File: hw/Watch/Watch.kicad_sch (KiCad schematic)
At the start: 8 parts, among them J3 Conn_01x02, J4 Conn_01x02, J5 Conn_01x02, J6 Conn_01x02

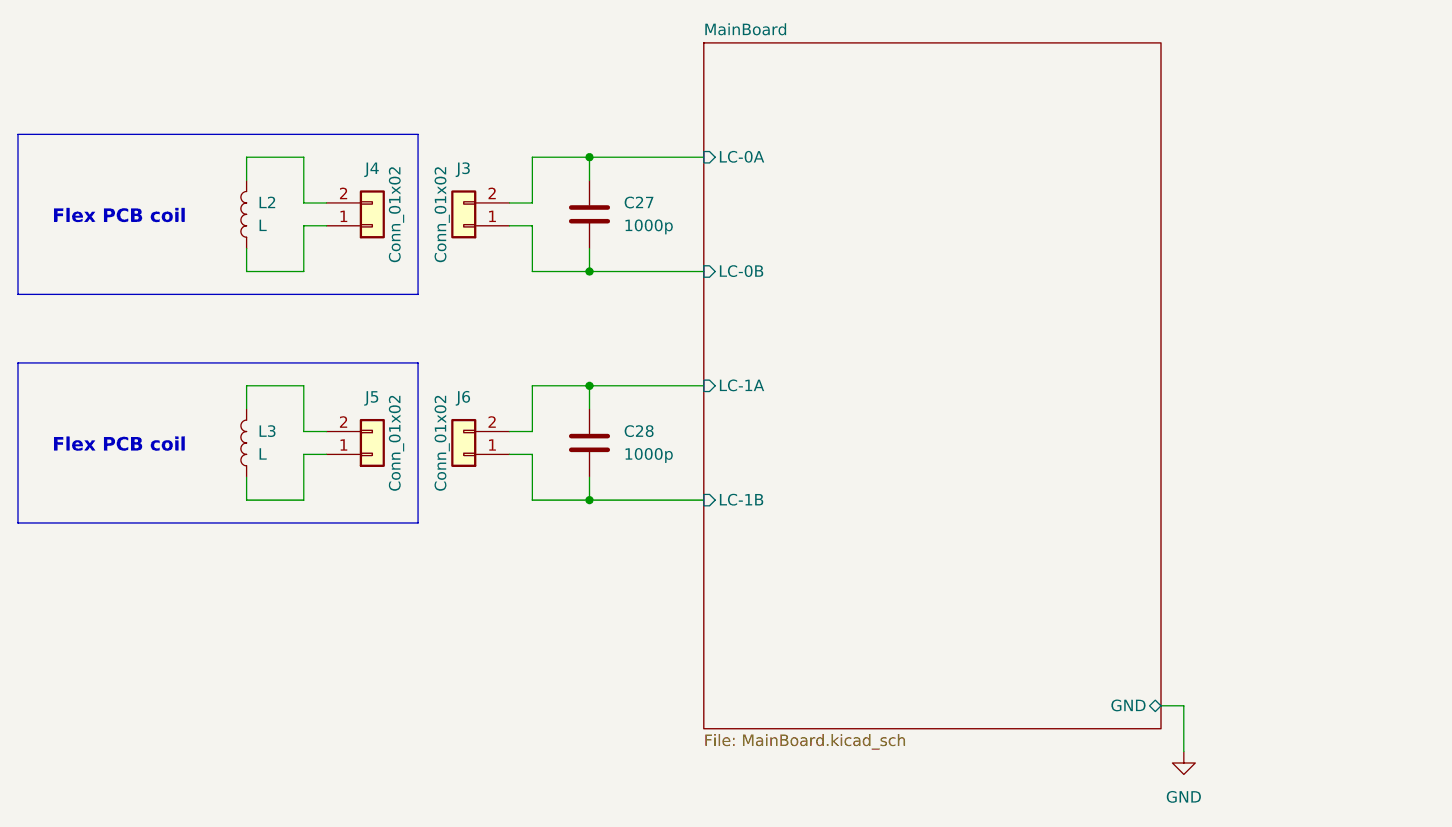
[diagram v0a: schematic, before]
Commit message: wip
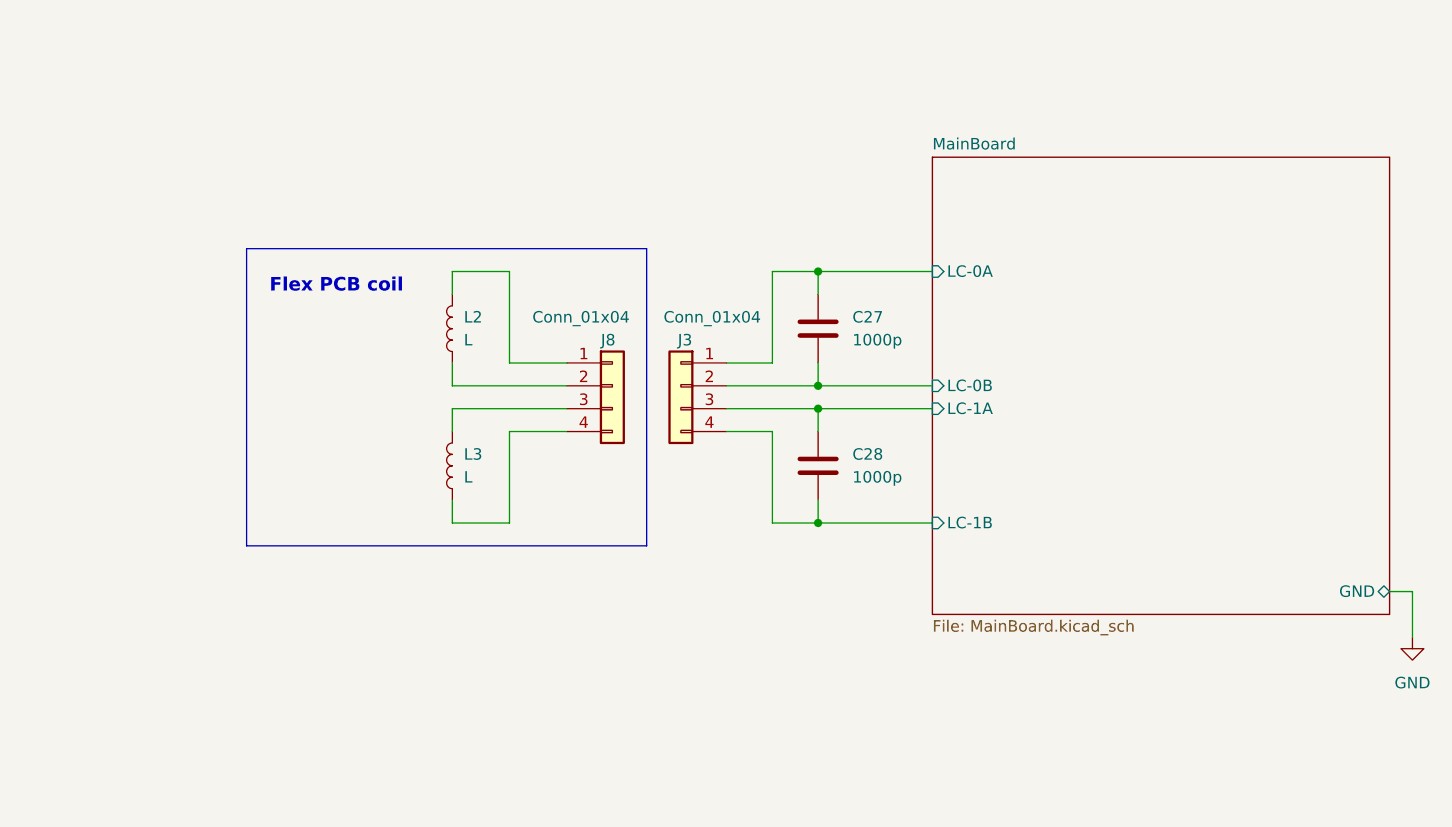
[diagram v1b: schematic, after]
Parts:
- removed J3, J4, J5, J6: Conn_01x02, symbol Connector_Generic:Conn_01x02
- added J3: Conn_01x04, RKL-Connectors:FFC-FPC_1x04_0.5mm, symbol Connector_Generic:Conn_01x04
- added J8: Conn_01x04, RKL-Connectors:FFC-FPC_1x04_0.5mm_cable, symbol Connector_Generic:Conn_01x04
- C27, C28: footprint Capacitor_SMD:C_0402_1005Metric -> Capacitor_SMD:C_0201_0603Metric; Basic/Extended B -> E; LCSC C1523 -> C66942
- L2, L3: footprint RKL-Inductors:PCB_coil -> RKL-Inductors:PCB_coil_linear_N24
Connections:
- net MainBoard/LC-0A: now also J3.1 (Pin_1)
- net MainBoard/LC-0B: now also J3.2 (Pin_2)
- net MainBoard/LC-1A: now also J3.3 (Pin_3)
- net MainBoard/LC-1B: now also J3.4 (Pin_4)
- net at L3.1: now also J8.3 (Pin_3)
- net at L3.2: now also J8.4 (Pin_4)
- net at L2.1: now also J8.1 (Pin_1)
- net at L2.2: now also J8.2 (Pin_2)
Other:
- moved on the sheet: C27, C28, L2, L3
